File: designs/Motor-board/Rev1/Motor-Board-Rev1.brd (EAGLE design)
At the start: 58.4 x 75 mm, 75 parts, among them IC1 REG1117, IC2 PIC16F1517/19PT

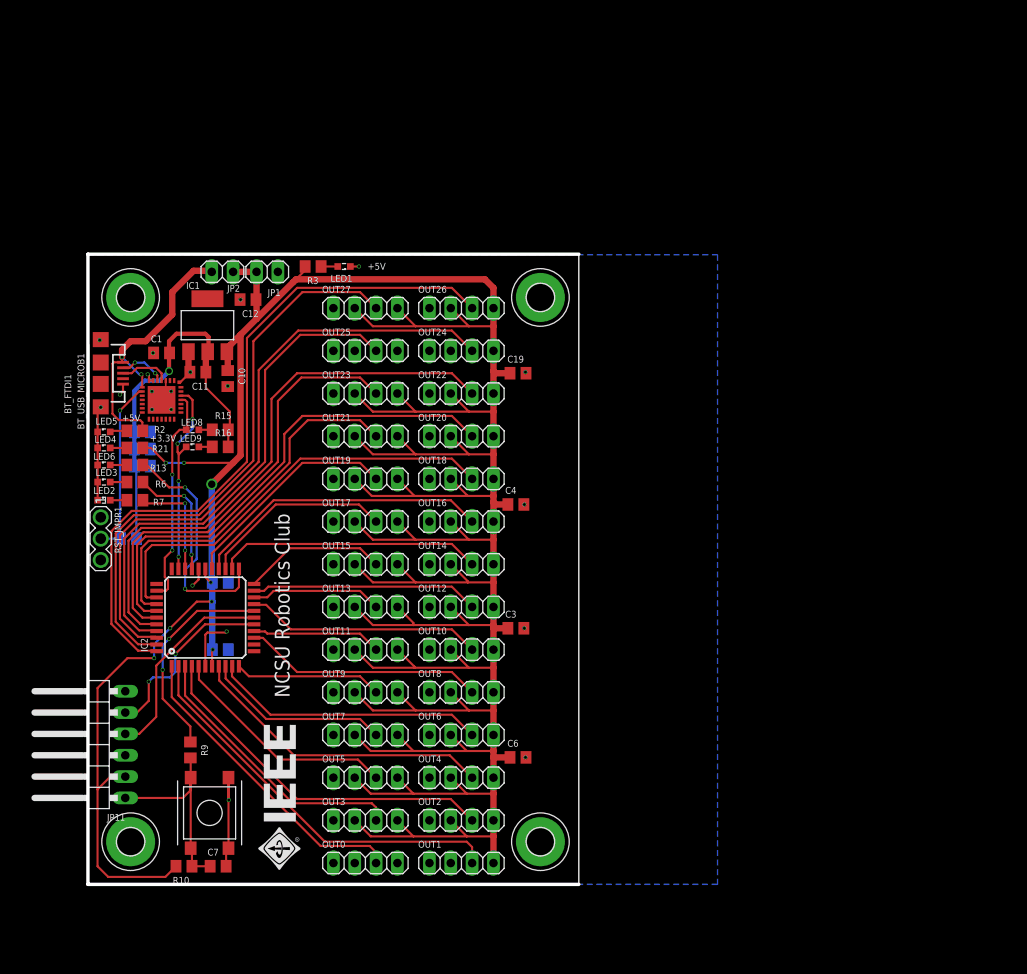
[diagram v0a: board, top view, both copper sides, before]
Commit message: done with first version of the boards
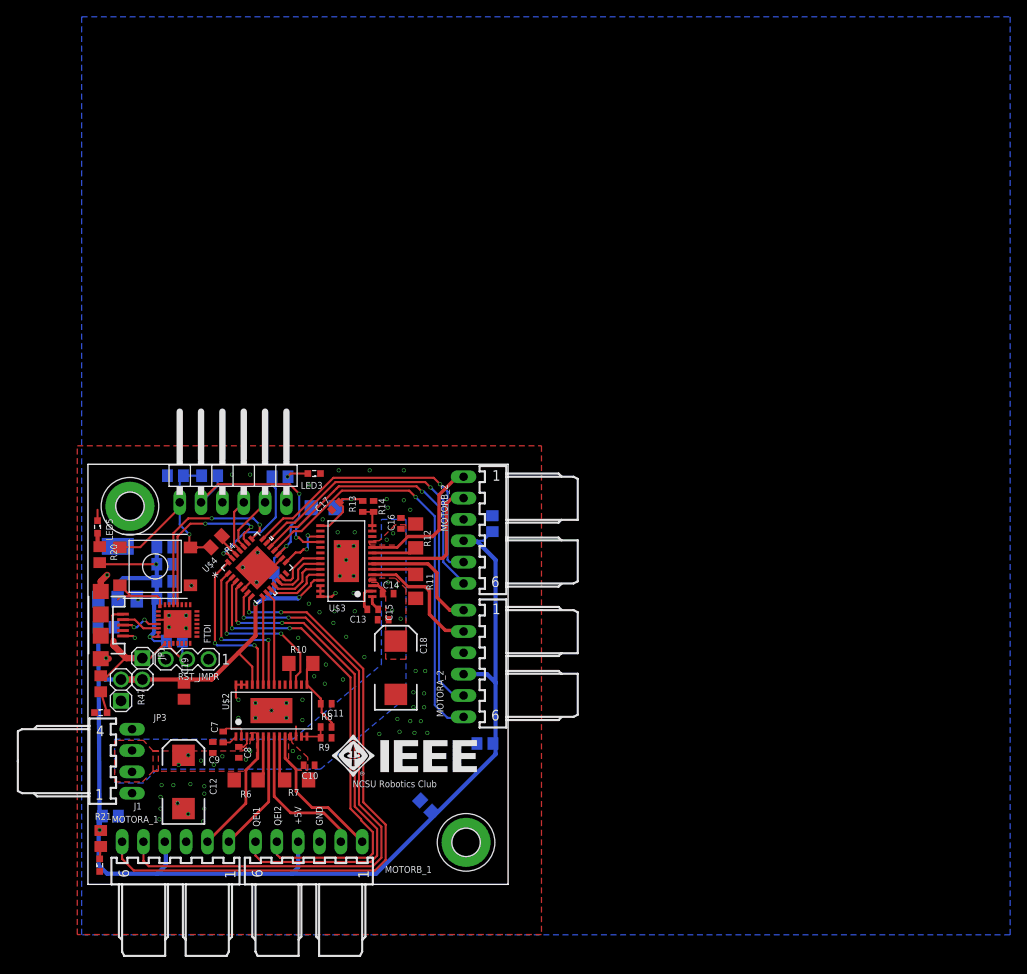
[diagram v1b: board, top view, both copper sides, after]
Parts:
- removed BT_FTDI1: CP2102, silabs:MLP28
- removed C4: 4.7uF, rcl:C0805
- removed H2, H4: MOUNT-PAD-ROUND3.2, holes:3,2-PAD
- removed IC1: REG1117, burr-brown:SOT223
- removed IC2: PIC16F1517/19PT, microchip:TQFP44
- removed JP2: (no value), pinhead:1X02
- removed LED1, LED2, LED6, LED8, LED9: (no value), interface_board-rev13:SML0603
- removed OUT0, OUT1, OUT10, OUT11, OUT12, OUT13, OUT14, OUT15, OUT16, OUT17, OUT18, OUT19, OUT2, OUT20, OUT21, OUT22, OUT23, OUT24, OUT25, OUT26, OUT27, OUT3, OUT4, OUT5, OUT6, OUT7, OUT8, OUT9: (no value), pinhead:1X04
- removed R16, R2, R3: 500, rcl:R0805
- removed RST_JMPR1: (no value), con-lstb:MA03-1
- added C13, C15, C16, C17: 0.1uF, rcl:C0402
- added C14: 0.47uF, rcl:C0402
- added C18: 100uF, SparkFun-Capacitors:EIA7343
- added C21: 4.7 uF, rcl:C0805
- added C37: 1uF, resistor:C0805
- added C38, C39: 0.1uF, resistor:C0805
- added C40: 4.7uF, resistor:C0805
- added FTDI: CP2102, silabs:MLP28
- added IC4: REG1117, burr-brown:SOT223
- added J1: 22-05-7048-04, con-molex:7395-04
- added JP3: (no value), pinhead:1X02
- added LED10: (no value), interface_board-rev13:SML0603
- added MOTORA_1, MOTORA_2, MOTORB_1, MOTORB_2: 22-05-7068-06, con-molex:7395-06
- added R11, R12: 0.1, rcl:R1206
- added R14: 15k, rcl:R0402
- added R20, R5: 10K, rcl:R0805
- added R4: 100, rcl:R0805
- added R46: 1k, resistor:R0805
- added R47: 500, resistor:R0805
- added R8: 10k, rcl:R0402
- added RST_JMPR: (no value), con-lstb:MA03-1
- added U$2, U$3: DRV8881PPWPR, motor-driver:TSSOP-28
- added U$4: PIC16F72-I/ML, Microchip_By_element14_Batch_1:QFN65P600X600X100-28N
- C1, C20, C5: value 1uF -> 0.1uF
- C10: value 10uF -> 0.1uF; device rcl:C0805 -> rcl:C0402
- C11, C9: value 4.7uF -> 0.1uF; device rcl:C0805 -> rcl:C0402
- C12: value 10uF -> 100uF; device rcl:C0805 -> SparkFun-Capacitors:EIA7343
- C3, C6: value 4.7uF -> 0.1uF
- C7: device rcl:C0805 -> rcl:C0402
- C8: value 0.1uF -> 0.47uF; device rcl:C0805 -> rcl:C0402
- R1: value 1k -> 10K; device resistor:R0805 -> rcl:R0805
- R10: device rcl:R0805 -> rcl:R1206
- R13: value 500 -> 10k; device rcl:R0805 -> rcl:R0402
- R15: value 500 -> 10K; device rcl:R0805 -> rcl:R1206
- R21: value 500 -> 10K
- R6, R7: value 500 -> 0.1; device rcl:R0805 -> rcl:R1206
- R9: value 100 -> 15k; device rcl:R0805 -> rcl:R0402
- moved H1 65.5 mm to (45.0, 5.00)
- moved C1 62.4 mm to (40.2, 9.31), flipped to the bottom, turned to 45 degrees
- moved C12 57.9 mm to (11.4, 12.2), turned to 90 degrees
- moved C19 54.9 mm to (11.4, 23.0), turned to 270 degrees
- moved LED4 49.7 mm to (1.40, 2.29), turned to 90 degrees
- moved JP1 49.5 mm to (6.48, 25.7), turned to 270 degrees
- moved C10 47.0 mm to (26.3, 14.2), turned to 0 degrees
- moved R21 46.7 mm to (1.52, 5.46), turned to 90 degrees
- moved C3 44.4 mm to (10.4, 48.6), flipped to the bottom
- moved C2 43.1 mm to (48.1, 42.9), turned to 90 degrees
- moved C11 42.3 mm to (28.4, 21.5), turned to 0 degrees
- moved H3 39.9 mm to (5.00, 45.0)
- moved R7 38.5 mm to (24.8, 12.4)
- moved R6 37.8 mm to (18.8, 12.4), turned to 180 degrees
- moved JP11 36.6 mm to (17.3, 49.3), turned to 0 degrees
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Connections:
- removed net ADC_1: IC2.1, OUT0.3
- removed net ADC_10: IC2.11, OUT9.3
- removed net ADC_11: IC2.19, OUT10.3
- removed net ADC_12: IC2.15, OUT11.3
- removed net ADC_13: IC2.21, OUT12.3
- removed net ADC_14: IC2.20, OUT13.3
- removed net ADC_15: IC2.24, OUT14.3
- removed net ADC_16: IC2.22, OUT15.3
- removed net ADC_17: IC2.26, OUT16.3
- removed net ADC_18: IC2.25, OUT17.3
- removed net ADC_19: IC2.36, OUT18.3
- removed net ADC_2: IC2.2, OUT1.3
- removed net ADC_20: IC2.27, OUT19.3
- removed net ADC_21: IC2.38, OUT20.3
- removed net ADC_22: IC2.37, OUT21.3
- removed net ADC_23: IC2.40, OUT22.3
- removed net ADC_24: IC2.39, OUT23.3
- removed net ADC_25: IC2.42, OUT24.3
- removed net ADC_26: IC2.41, OUT25.3
- removed net ADC_27: IC2.44, OUT26.3
- removed net ADC_28: IC2.43, OUT27.3
- removed net ADC_3: IC2.4, OUT2.3
- removed net ADC_4: IC2.3, OUT3.3
- removed net ADC_5: IC2.8, OUT4.3
- removed net ADC_6: IC2.5, OUT5.3
- removed net ADC_7: IC2.10, OUT6.3
- removed net ADC_8: IC2.9, OUT7.3
- removed net ADC_9: IC2.14, OUT8.3
- removed net BT_D+1: BT_FTDI1.4, BT_USB_MICROB1.D+
- removed net BT_D-1: BT_FTDI1.5, BT_USB_MICROB1.D-
- removed net N$12: LED5.A, R2.1
- removed net N$2: BT_FTDI1.9, R1.1, RST_JMPR1.2
- removed net N$3: LED6.A, R13.1
- removed net N$6: LED2.A, R7.1
- removed net STATUS_0: IC2.23, R13.2
- removed net STATUS_1: IC2.30, R6.2
- removed net STATUS_2: IC2.31, R7.2
- removed net UART_RX: BT_FTDI1.26, IC2.32, LED9.C
- removed net UART_TX: BT_FTDI1.25, IC2.35, LED8.C
- new net +7V: C10.1, C12.A, C14.2, C15.1, C16.1, C18.A, C8.2, C9.1, J1.2, J1.3, U$2.11, U$2.4, U$3.11, U$3.4
- new net AEN_1: U$2.23, U$4.8
- new net AEN_2: U$3.23, U$4.11
- new net APH_1: U$2.24, U$4.28
- new net APH_2: U$3.24, U$4.10
- new net BEN_1: U$2.21, U$4.9
- new net BEN_2: U$3.21, U$4.13
- new net BPH_1: U$2.22, U$4.1
- new net BPH_2: U$3.22, U$4.12
- new net BT_D+: BT_USB_MICROB1.D+, FTDI.4
- new net BT_D-: BT_USB_MICROB1.D-, FTDI.5
- new net MOTOR1A_1: MOTORA_1.2, U$2.5
- new net MOTOR1A_2: MOTORA_1.1, U$2.7
- new net MOTOR1B_1: MOTORB_1.2, U$2.8
- new net MOTOR1B_2: MOTORB_1.1, U$2.10
- new net MOTOR2A_1: MOTORA_2.2, U$3.5
- new net MOTOR2A_2: MOTORA_2.1, U$3.7
- new net MOTOR2B_1: MOTORB_2.2, U$3.8
- new net MOTOR2B_2: MOTORB_2.1, U$3.10
- new net N$16: C7.2, U$2.2
- new net N$17: C7.1, U$2.1
- new net N$19: C8.1, U$2.3
- new net N$20: R8.2, R9.1, U$2.13, U$2.14
- new net N$21: R12.1, U$3.9
- new net N$22: R11.1, U$3.6
- new net N$27: C13.2, U$3.2
- new net N$28: C13.1, U$3.1
- new net N$29: C14.1, U$3.3
- new net N$30: R13.2, R14.1, U$3.13, U$3.14
- new net N$5: LED5.A, R20.1
- new net N$9: FTDI.9, R46.1, RST_JMPR.2
- new net NFAULT_1: R10.1, U$2.18
- new net NFAULT_2: R15.1, U$3.18
- new net NSLEEP_1: U$2.17, U$4.2
- new net NSLEEP_2: U$3.17, U$4.15
- new net QEIA1_1: MOTORA_1.5, U$4.6
- new net QEIA1_2: MOTORA_1.6, U$4.7
- new net QEIA2_1: MOTORA_2.5, U$4.19
- new net QEIA2_2: MOTORA_2.6, U$4.18
- new net QEIB1_1: MOTORB_1.5, U$4.3
- new net QEIB1_2: MOTORB_1.6, U$4.4
- new net QEIB2_1: MOTORB_2.5, U$4.21
- new net QEIB2_2: MOTORB_2.6, U$4.20
- new net RX: FTDI.26, U$4.22
- new net STATUS1: R1.2, U$4.27
- new net TX: FTDI.25, U$4.23
- new net V3P3_1: C11.1, R10.2, R8.1, U$2.15
- new net V3P3_2: C17.1, R13.1, R15.2, U$3.15
- net +3V3: now also C37.2, C38.2, C39.2, C40.2, FTDI.6, FTDI.7, IC4.2, R20.2, R46.2; no longer BT_FTDI1.6, BT_FTDI1.7, C1.2, C11.1, C2.2, C8.2, C9.2, IC1.2, R1.2, R15.2, R16.2
- net +5V: now also C1.1, C2.1, C21.1, IC4.3, JP1.2, JP3.2, MOTORA_1.4, MOTORA_2.4, MOTORB_1.4, MOTORB_2.4, R5.2, U$2.25, U$3.25, U$4.17; no longer C10.1, C12.1, C3.1, C4.1, IC1.3, IC2.28, IC2.7, JP1.1, JP2.2, OUT0.2, OUT0.4, OUT1.2, OUT1.4, OUT10.2, OUT10.4, OUT11.2, OUT11.4, OUT12.2, OUT12.4, OUT13.2, OUT13.4, OUT14.2, OUT14.4, OUT15.2, OUT15.4, OUT16.2, OUT16.4, OUT17.2, OUT17.4, OUT18.2, OUT18.4, OUT19.2, OUT19.4, OUT2.2, OUT2.4, OUT20.2, OUT20.4, OUT21.2, OUT21.4, OUT22.2, OUT22.4, OUT23.2, OUT23.4, OUT24.2, OUT24.4, OUT25.2, OUT25.4, OUT26.2, OUT26.4, OUT27.2, OUT27.4, OUT3.2, OUT3.4, OUT4.2, OUT4.4, OUT5.2, OUT5.4, OUT6.2, OUT6.4, OUT7.2, OUT7.4, OUT8.2, OUT8.4, OUT9.2, OUT9.4, R10.2, R3.2
- net GND: now also C1.2, C12.C, C15.2, C16.2, C17.2, C18.C, C2.2, C21.2, C37.1, C38.1, C39.1, C40.1, C9.2, FTDI.3, FTDI.EXP, FTDI.M, IC4.1, J1.1, J1.4, JP3.1, LED10.C, MOTORA_1.3, MOTORA_2.3, MOTORB_1.3, MOTORB_2.3, R11.2, R12.2, R14.2, R6.2, R7.2, R9.2, RST_JMPR.3, U$2.12, U$2.26, U$2.27, U$2.28, U$2.EXP, U$3.12, U$3.26, U$3.27, U$3.28, U$3.EXP, U$4.16, U$4.29, U$4.5; no longer BT_FTDI1.3, BT_FTDI1.EXP, BT_FTDI1.M, C1.1, C12.2, C2.1, C4.2, C7.2, C8.1, C9.1, H2.B3,2, H4.B3,2, IC1.1, IC2.29, IC2.6, JP1.2, LED1.C, LED2.C, LED6.C, OUT0.1, OUT1.1, OUT10.1, OUT11.1, OUT12.1, OUT13.1, OUT14.1, OUT15.1, OUT16.1, OUT17.1, OUT18.1, OUT19.1, OUT2.1, OUT20.1, OUT21.1, OUT22.1, OUT23.1, OUT24.1, OUT25.1, OUT26.1, OUT27.1, OUT3.1, OUT4.1, OUT5.1, OUT6.1, OUT7.1, OUT8.1, OUT9.1, RST_JMPR1.3
- net ICDCLK: now also U$4.24; no longer IC2.16
- net ICDDAT: now also U$4.25; no longer IC2.17
- net MCLR: now also C3.1, R4.2, R5.1; no longer C7.1, R10.1, R9.2
- net MCLR`: now also R4.1, U$4.26; no longer IC2.18, R9.1
- net N$1: now also R1.1; no longer R6.1
- net N$10: now also LED10.A, R47.1; no longer LED8.A, R15.1
- net N$11: now also R6.1, U$2.6; no longer LED9.A, R16.1
- net N$4: now also R7.1, U$2.9; no longer LED1.A, R3.1
- net NC_1_FTDI: now also FTDI.12; no longer BT_FTDI1.12
- net NC_2_FTDI: now also FTDI.11; no longer BT_FTDI1.11
- net NC_3_FTDI: now also FTDI.2; no longer BT_FTDI1.2
- net NC_4_FTDI: now also FTDI.1; no longer BT_FTDI1.1
- net NC_5_FTDI: now also FTDI.28; no longer BT_FTDI1.28
- net NC_6_FTDI: now also FTDI.27; no longer BT_FTDI1.27
- net NC_7_FTDI: now also FTDI.24; no longer BT_FTDI1.24
- net NC_8_FTDI: now also FTDI.23; no longer BT_FTDI1.23
- net VBUS: now also FTDI.8, JP1.1, R47.2; no longer BT_FTDI1.8, JP2.1, R2.2
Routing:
- net +5V: track 513.2 -> 205.5 mm, vias 8 -> 5
- net ADC_27: track 82.3 -> 0.00 mm
- net QEIA1_2: track 0.00 -> 76.7 mm, vias 0 -> 2
- net ADC_25: track 74.6 -> 0.00 mm
- net QEIA1_1: track 0.00 -> 74.1 mm, vias 0 -> 2
- net ADC_28: track 68.5 -> 0.00 mm
- net ADC_23: track 67.0 -> 0.00 mm
- net ADC_26: track 61.0 -> 0.00 mm
- net QEIB1_2: track 0.00 -> 60.6 mm, vias 0 -> 2
- net ADC_21: track 58.9 -> 0.00 mm
- net QEIB1_1: track 0.00 -> 57.7 mm, vias 0 -> 2
- net ADC_24: track 53.2 -> 0.00 mm
- net ADC_19: track 51.2 -> 0.00 mm
- net QEIA2_2: track 0.00 -> 49.9 mm, vias 0 -> 1
- net QEIA2_1: track 0.00 -> 48.4 mm, vias 0 -> 1
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- added copper zone on layer 1, net +7V
- added copper zone on layer 16, net +7V
- added copper zone on layer 1, net GND
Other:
- board size 58.4 x 75 mm -> 50 x 50 mm
- board text added: "GND"
- board text added: "QEI1"
- board text added: "QEI2"
- board text removed: "+3.3V"
